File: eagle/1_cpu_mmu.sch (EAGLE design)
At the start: 28 parts, among them IC1 MT5C6408, IC10 74LS157N, IC11 74LS157N, IC12 74LS00N, IC13 74LS157N, IC14 74LS157N, IC15 74LS04N, IC19 74LS32N, IC2 MT5C6408, IC20 74LS02N, IC21 74LS374N, IC3 74LS27N, IC4 74LS20N, IC5 74LS08N, IC6 74LS245N, IC7 74LS245N, IC8 74LS32N, IC9 74LS157N

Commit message: MMU schematics completed
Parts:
- removed IC15: 74LS04N, 74xx-eu:74LS04N
- added IC16: 74LS08N, 74xx-eu:74LS08N
- added IC17: 74LS32N, 74xx-eu:74LS32N
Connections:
- removed net FIO: IC15B.I, IC2G$1.DQ6, IC7A.A6
- removed net FPRESENT: IC2G$1.DQ8, IC7A.A8
- removed net FWRITABLE: IC2G$1.DQ7, IC7A.A7
- removed net N$18: IC11A.3A, IC15B.O
- removed net N$19: IC12A.I1
- removed net N$31: IC12A.I0
- new net /FIO: IC11A.3A, IC2G$1.DQ6, IC7A.A6
- new net /FPRESENT: IC12B.I0, IC2G$1.DQ8, IC7A.A8
- new net /FWRITABLE: IC12D.I0, IC2G$1.DQ7, IC7A.A7
- new net N$33: IC12B.I1, IC20A.O, IC5B.I0
- new net N$34: IC12D.I1, IC5B.O
- net /ENMEM: now also IC17A.I1, IC5B.I1
- net /ENMEMX: now also IC17A.O
- net /FP: now also IC17C.I1; no longer IC19A.I1
- net /LDMEM: now also IC17B.I1
- net /LDMEMX: now also IC17B.O
- net /MEMOP: now also IC17C.I0; no longer IC19A.I0
- net /NP_FAULT: now also IC12B.O, IC16B.I0
- net /WR_FAULT: now also IC12D.O, IC16B.I1
- net ABUS0: now also IC12A.I1; no longer IC15A.I
- net GND: no longer IC10A.2B
- net MEMSEG: now also IC10A.2B
- net N$20: now also IC17C.O, IC20A.I0; no longer IC19A.O, IC19B.I0
- net N$30: now also IC12A.O; no longer IC15A.O
- net N$32: now also IC17A.I0, IC17B.I0, IC20A.I1; no longer IC19B.I1
- net N$40: now also IC16B.O; no longer IC12A.O
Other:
- moved on the sheet: IC12A, IC12C, IC19C, IC19D, IC21

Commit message: MMU power rails and bypass caps added in schematic, board started
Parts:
- added C1, C10, C11, C12, C13, C14, C15, C16, C17, C19, C2, C3, C4, C5, C6, C7, C8, C9: 100n, rcl:C-EU050-024X044
- added C18: 10u, rcl:CPOL-EUE2.5-6
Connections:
- net +5V: now also C1.1, C10.1, C11.1, C12.1, C13.1, C14.1, C15.1, C16.1, C17.1, C18.+, C19.1, C2.1, C3.1, C4.1, C5.1, C6.1, C7.1, C8.1, C9.1, IC10P.VCC, IC11P.VCC, IC12P.VCC, IC13P.VCC, IC14P.VCC, IC16P.VCC, IC17P.VCC, IC19P.VCC, IC1P.VCC, IC20P.VCC, IC21P.VCC, IC2P.VCC, IC3P.VCC, IC4P.VCC, IC5P.VCC, IC6P.VCC, IC7P.VCC, IC9P.VCC
- net GND: now also C1.2, C10.2, C11.2, C12.2, C13.2, C14.2, C15.2, C16.2, C17.2, C18.-, C19.2, C2.2, C3.2, C4.2, C5.2, C6.2, C7.2, C8.2, C9.2, IC10P.GND, IC11P.GND, IC12P.GND, IC13P.GND, IC14P.GND, IC16A.I0, IC16A.I1, IC16C.I0, IC16C.I1, IC16D.I0, IC16D.I1, IC16P.GND, IC17D.I0, IC17D.I1, IC17P.GND, IC19A.I0, IC19A.I1, IC19B.I0, IC19B.I1, IC19P.GND, IC1P.GND, IC20C.I0, IC20C.I1, IC20D.I0, IC20D.I1, IC20P.GND, IC21P.GND, IC2P.GND, IC3P.GND, IC4P.GND, IC5P.GND, IC6P.GND, IC7P.GND, IC9P.GND

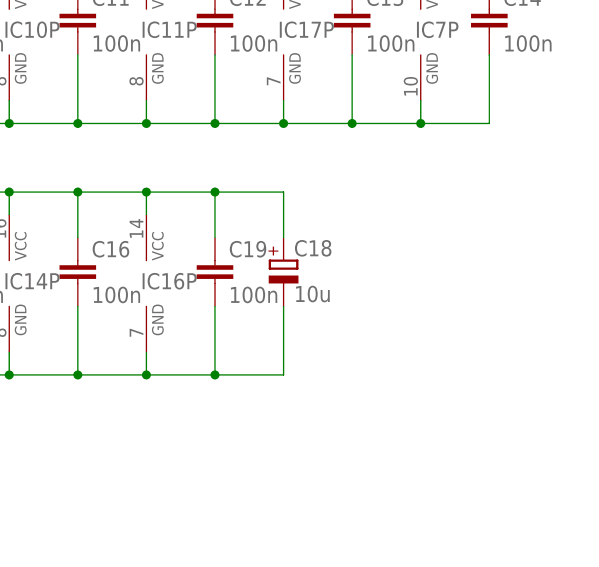
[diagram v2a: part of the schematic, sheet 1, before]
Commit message: MMU board updates 2016-02-25
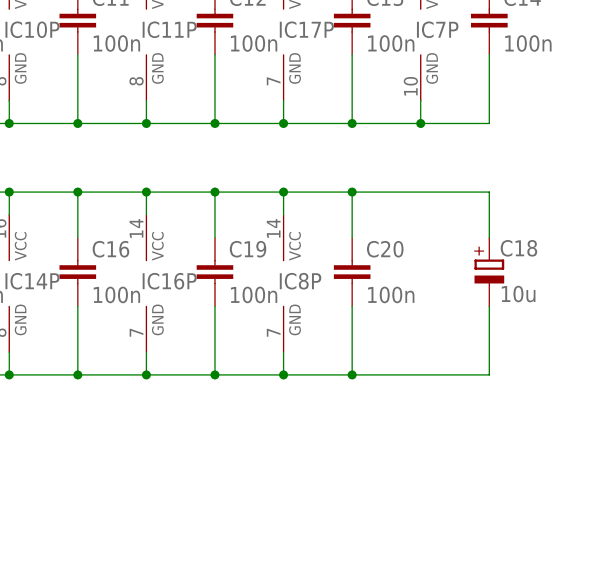
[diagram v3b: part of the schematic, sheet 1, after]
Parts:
- added C20: 100n, rcl:C-EU050-024X044
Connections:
- net +5V: now also C20.1, IC8P.VCC
- net GND: now also C20.2, IC8P.GND
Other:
- moved on the sheet: C18
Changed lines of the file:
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@@
 <part name="SUPPLY18" library="supply2" deviceset="+5V" device=""/>
 <part name="SUPPLY19" library="supply2" deviceset="+5V" device=""/>
+<part name="C20" library="rcl" deviceset="C-EU" device="050-024X044" value="100n"/>
 </parts>
 <sheets>
@@
 <instance part="IC21" gate="P" x="368.3" y="248.92"/>
 <instance part="C17" gate="G$1" x="330.2" y="251.46"/>
-<instance part="C18" gate="G$1" x="353.06" y="167.64"/>
+<instance part="C18" gate="G$1" x="375.92" y="167.64"/>
 <instance part="C1" gate="G$1" x="314.96" y="251.46"/>
 <instance part="SUPPLY12" gate="GND" x="302.26" y="154.94" rot="R270"/>
@@
 <instance part="SUPPLY18" gate="+5V" x="302.26" y="203.2" rot="R90"/>
 <instance part="SUPPLY19" gate="+5V" x="302.26" y="175.26" rot="R90"/>
+<instance part="IC8" gate="P" x="353.06" y="165.1"/>
+<instance part="C20" gate="G$1" x="360.68" y="167.64"/>
 </instances>
 <busses>
@@
 <segment>
 <pinref part="SUPPLY12" gate="GND" pin="GND"/>
-<pinref part="C18" gate="G$1" pin="-"/>
 <wire x1="304.8" y1="154.94" x2="307.34" y2="154.94" width="0.1524" layer="91"/>
 <wire x1="307.34" y1="154.94" x2="314.96" y2="154.94" width="0.1524" layer="91"/>
@@
 <wire x1="330.2" y1="154.94" x2="337.82" y2="154.94" width="0.1524" layer="91"/>
 <wire x1="337.82" y1="154.94" x2="345.44" y2="154.94" width="0.1524" layer="91"/>
-<wire x1="345.44" y1="154.94" x2="353.06" y2="154.94" width="0.1524" layer="91"/>
-<wire x1="353.06" y1="154.94" x2="353.06" y2="162.56" width="0.1524" layer="91"/>
 <pinref part="C19" gate="G$1" pin="2"/>
 <wire x1="345.44" y1="162.56" x2="345.44" y2="154.94" width="0.1524" layer="91"/>
@@
 <junction x="314.96" y="154.94"/>
 <junction x="307.34" y="154.94"/>
+<pinref part="C18" gate="G$1" pin="-"/>
+<wire x1="345.44" y1="154.94" x2="353.06" y2="154.94" width="0.1524" layer="91"/>
+<wire x1="353.06" y1="154.94" x2="360.68" y2="154.94" width="0.1524" layer="91"/>
+<wire x1="360.68" y1="154.94" x2="375.92" y2="154.94" width="0.1524" layer="91"/>
+<wire x1="375.92" y1="154.94" x2="375.92" y2="162.56" width="0.1524" layer="91"/>
+<pinref part="IC8" gate="P" pin="GND"/>
+<wire x1="353.06" y1="154.94" x2="353.06" y2="157.48" width="0.1524" layer="91"/>
+<pinref part="C20" gate="G$1" pin="2"/>
+<wire x1="360.68" y1="154.94" x2="360.68" y2="162.56" width="0.1524" layer="91"/>
+<junction x="353.06" y="154.94"/>
+<junction x="360.68" y="154.94"/>
 </segment>
 <segment>
@@
 </segment>
 <segment>
-<pinref part="C18" gate="G$1" pin="+"/>
-<wire x1="353.06" y1="170.18" x2="353.06" y2="175.26" width="0.1524" layer="91"/>
 <pinref part="SUPPLY19" gate="+5V" pin="+5V"/>
-<wire x1="353.06" y1="175.26" x2="345.44" y2="175.26" width="0.1524" layer="91"/>
 <pinref part="IC13" gate="P" pin="VCC"/>
 <wire x1="345.44" y1="175.26" x2="337.82" y2="175.26" width="0.1524" layer="91"/>
@@
 <junction x="337.82" y="175.26"/>
 <junction x="345.44" y="175.26"/>
-</segment>
-<segment>
+<pinref part="C18" gate="G$1" pin="+"/>
+<wire x1="375.92" y1="170.18" x2="375.92" y2="175.26" width="0.1524" layer="91"/>
+<wire x1="375.92" y1="175.26" x2="360.68" y2="175.26" width="0.1524" layer="91"/>
+<pinref part="IC8" gate="P" pin="VCC"/>
+<wire x1="360.68" y1="175.26" x2="353.06" y2="175.26" width="0.1524" layer="91"/>
+<wire x1="353.06" y1="175.26" x2="345.44" y2="175.26" width="0.1524" layer="91"/>
+<wire x1="353.06" y1="172.72" x2="353.06" y2="175.26" width="0.1524" layer="91"/>
+<pinref part="C20" gate="G$1" pin="1"/>
+<wire x1="360.68" y1="170.18" x2="360.68" y2="175.26" width="0.1524" layer="91"/>
+<junction x="353.06" y="175.26"/>
+<junction x="360.68" y="175.26"/>
+</segment>
+<segment>
